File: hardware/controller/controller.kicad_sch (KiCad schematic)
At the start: 4 parts

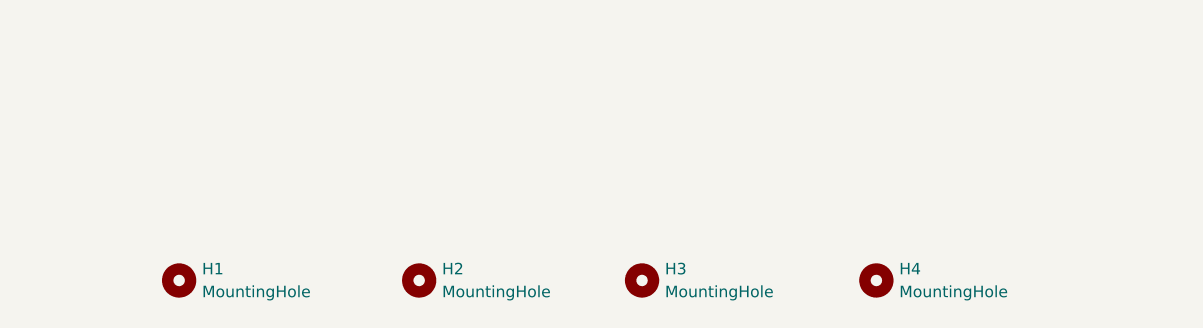
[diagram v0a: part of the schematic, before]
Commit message: hooking up parts in the schematic
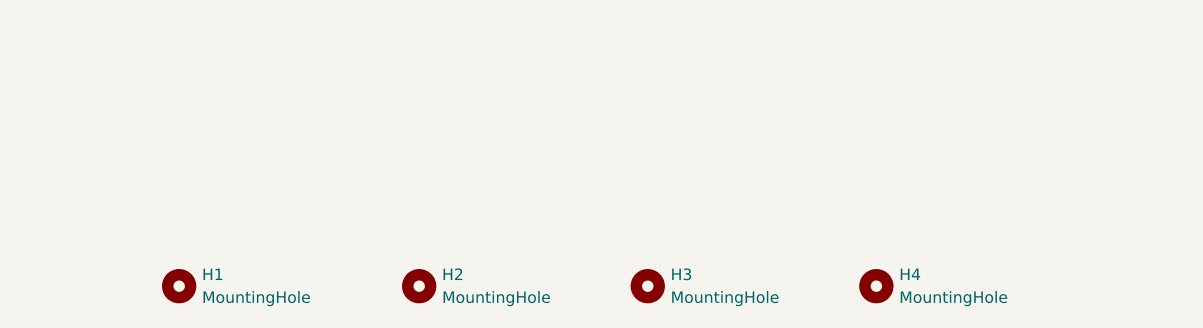
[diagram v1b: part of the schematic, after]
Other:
- moved on the sheet: H1, H2, H3, H4
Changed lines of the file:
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@@
 	(symbol
 		(lib_id "Mechanical:MountingHole")
-		(at 48.26 102.235 0)
+		(at 48.26 102.87 0)
 		(unit 1)
 		(body_style 1)
@@
 		(fields_autoplaced yes)
 		(property "Reference" "H1"
-			(at 50.8 100.9649 0)
-			(show_name no)
-			(do_not_autoplace no)
-			(effects
-				(font
-					(size 1.27 1.27)
-				)
-				(justify left)
-			)
-		)
-		(property "Value" "MountingHole"
-			(at 50.8 103.5049 0)
-			(show_name no)
-			(do_not_autoplace no)
-			(effects
-				(font
-					(size 1.27 1.27)
-				)
-				(justify left)
-			)
-		)
-		(property "Footprint" "MountingHole:MountingHole_3.2mm_M3_Pad"
-			(at 48.26 102.235 0)
-			(hide yes)
-			(show_name no)
-			(do_not_autoplace no)
-			(effects
-				(font
-					(size 1.27 1.27)
-				)
-			)
-		)
-		(property "Datasheet" ""
-			(at 48.26 102.235 0)
-			(hide yes)
-			(show_name no)
-			(do_not_autoplace no)
-			(effects
-				(font
-					(size 1.27 1.27)
-				)
-			)
-		)
-		(property "Description" "Mounting Hole without connection"
-			(at 48.26 102.235 0)
+			(at 50.8 101.5999 0)
+			(show_name no)
+			(do_not_autoplace no)
+			(effects
+				(font
+					(size 1.27 1.27)
+				)
+				(justify left)
+			)
+		)
+		(property "Value" "MountingHole"
+			(at 50.8 104.1399 0)
+			(show_name no)
+			(do_not_autoplace no)
+			(effects
+				(font
+					(size 1.27 1.27)
+				)
+				(justify left)
+			)
+		)
+		(property "Footprint" "MountingHole:MountingHole_3.2mm_M3_Pad"
+			(at 48.26 102.87 0)
+			(hide yes)
+			(show_name no)
+			(do_not_autoplace no)
+			(effects
+				(font
+					(size 1.27 1.27)
+				)
+			)
+		)
+		(property "Datasheet" ""
+			(at 48.26 102.87 0)
+			(hide yes)
+			(show_name no)
+			(do_not_autoplace no)
+			(effects
+				(font
+					(size 1.27 1.27)
+				)
+			)
+		)
+		(property "Description" "Mounting Hole without connection"
+			(at 48.26 102.87 0)
 			(hide yes)
 			(show_name no)
@@
 	(symbol
 		(lib_id "Mechanical:MountingHole")
-		(at 125.73 102.235 0)
+		(at 125.73 102.87 0)
 		(unit 1)
 		(body_style 1)
@@
 		(fields_autoplaced yes)
 		(property "Reference" "H4"
-			(at 128.27 100.9649 0)
-			(show_name no)
-			(do_not_autoplace no)
-			(effects
-				(font
-					(size 1.27 1.27)
-				)
-				(justify left)
-			)
-		)
-		(property "Value" "MountingHole"
-			(at 128.27 103.5049 0)
-			(show_name no)
-			(do_not_autoplace no)
-			(effects
-				(font
-					(size 1.27 1.27)
-				)
-				(justify left)
-			)
-		)
-		(property "Footprint" "MountingHole:MountingHole_3.2mm_M3_Pad"
-			(at 125.73 102.235 0)
-			(hide yes)
-			(show_name no)
-			(do_not_autoplace no)
-			(effects
-				(font
-					(size 1.27 1.27)
-				)
-			)
-		)
-		(property "Datasheet" ""
-			(at 125.73 102.235 0)
-			(hide yes)
-			(show_name no)
-			(do_not_autoplace no)
-			(effects
-				(font
-					(size 1.27 1.27)
-				)
-			)
-		)
-		(property "Description" "Mounting Hole without connection"
-			(at 125.73 102.235 0)
+			(at 128.27 101.5999 0)
+			(show_name no)
+			(do_not_autoplace no)
+			(effects
+				(font
+					(size 1.27 1.27)
+				)
+				(justify left)
+			)
+		)
+		(property "Value" "MountingHole"
+			(at 128.27 104.1399 0)
+			(show_name no)
+			(do_not_autoplace no)
+			(effects
+				(font
+					(size 1.27 1.27)
+				)
+				(justify left)
+			)
+		)
+		(property "Footprint" "MountingHole:MountingHole_3.2mm_M3_Pad"
+			(at 125.73 102.87 0)
+			(hide yes)
+			(show_name no)
+			(do_not_autoplace no)
+			(effects
+				(font
+					(size 1.27 1.27)
+				)
+			)
+		)
+		(property "Datasheet" ""
+			(at 125.73 102.87 0)
+			(hide yes)
+			(show_name no)
+			(do_not_autoplace no)
+			(effects
+				(font
+					(size 1.27 1.27)
+				)
+			)
+		)
+		(property "Description" "Mounting Hole without connection"
+			(at 125.73 102.87 0)
 			(hide yes)
 			(show_name no)
@@
 	(symbol
 		(lib_id "Mechanical:MountingHole")
-		(at 74.93 102.235 0)
+		(at 74.93 102.87 0)
 		(unit 1)
 		(body_style 1)
@@
 		(fields_autoplaced yes)
 		(property "Reference" "H2"
-			(at 77.47 100.9649 0)
-			(show_name no)
-			(do_not_autoplace no)
-			(effects
-				(font
-					(size 1.27 1.27)
-				)
-				(justify left)
-			)
-		)
-		(property "Value" "MountingHole"
-			(at 77.47 103.5049 0)
-			(show_name no)
-			(do_not_autoplace no)
-			(effects
-				(font
-					(size 1.27 1.27)
-				)
-				(justify left)
-			)
-		)
-		(property "Footprint" "MountingHole:MountingHole_3.2mm_M3_Pad"
-			(at 74.93 102.235 0)
-			(hide yes)
-			(show_name no)
-			(do_not_autoplace no)
-			(effects
-				(font
-					(size 1.27 1.27)
-				)
-			)
-		)
-		(property "Datasheet" ""
-			(at 74.93 102.235 0)
-			(hide yes)
-			(show_name no)
-			(do_not_autoplace no)
-			(effects
-				(font
-					(size 1.27 1.27)
-				)
-			)
-		)
-		(property "Description" "Mounting Hole without connection"
-			(at 74.93 102.235 0)
+			(at 77.47 101.5999 0)
+			(show_name no)
+			(do_not_autoplace no)
+			(effects
+				(font
+					(size 1.27 1.27)
+				)
+				(justify left)
+			)
+		)
+		(property "Value" "MountingHole"
+			(at 77.47 104.1399 0)
+			(show_name no)
+			(do_not_autoplace no)
+			(effects
+				(font
+					(size 1.27 1.27)
+				)
+				(justify left)
+			)
+		)
+		(property "Footprint" "MountingHole:MountingHole_3.2mm_M3_Pad"
+			(at 74.93 102.87 0)
+			(hide yes)
+			(show_name no)
+			(do_not_autoplace no)
+			(effects
+				(font
+					(size 1.27 1.27)
+				)
+			)
+		)
+		(property "Datasheet" ""
+			(at 74.93 102.87 0)
+			(hide yes)
+			(show_name no)
+			(do_not_autoplace no)
+			(effects
+				(font
+					(size 1.27 1.27)
+				)
+			)
+		)
+		(property "Description" "Mounting Hole without connection"
+			(at 74.93 102.87 0)
 			(hide yes)
 			(show_name no)
@@
 	(symbol
 		(lib_id "Mechanical:MountingHole")
-		(at 99.695 102.235 0)
+		(at 100.33 102.87 0)
 		(unit 1)
 		(body_style 1)
@@
 		(fields_autoplaced yes)
 		(property "Reference" "H3"
-			(at 102.235 100.9649 0)
-			(show_name no)
-			(do_not_autoplace no)
-			(effects
-				(font
-					(size 1.27 1.27)
-				)
-				(justify left)
-			)
-		)
-		(property "Value" "MountingHole"
-			(at 102.235 103.5049 0)
-			(show_name no)
-			(do_not_autoplace no)
-			(effects
-				(font
-					(size 1.27 1.27)
-				)
-				(justify left)
-			)
-		)
-		(property "Footprint" "MountingHole:MountingHole_3.2mm_M3_Pad"
-			(at 99.695 102.235 0)
-			(hide yes)
-			(show_name no)
-			(do_not_autoplace no)
-			(effects
-				(font
-					(size 1.27 1.27)
-				)
-			)
-		)
-		(property "Datasheet" ""
-			(at 99.695 102.235 0)
-			(hide yes)
-			(show_name no)
-			(do_not_autoplace no)
-			(effects
-				(font
-					(size 1.27 1.27)
-				)
-			)
-		)
-		(property "Description" "Mounting Hole without connection"
-			(at 99.695 102.235 0)
-			(hide yes)
-			(show_name no)
+			(at 102.87 101.5999 0)
+			(show_name no)
+			(do_not_autoplace no)
+			(effects
+				(font
+					(size 1.27 1.27)
+				)
+				(justify left)
+			)
+		)
+		(property "Value" "MountingHole"
+			(at 102.87 104.1399 0)
+			(show_name no)
+			(do_not_autoplace no)
+			(effects
+				(font
+					(size 1.27 1.27)
+				)
+				(justify left)
+			)
+		)
+		(property "Footprint" "MountingHole:MountingHole_3.2mm_M3_Pad"
+			(at 100.33 102.87 0)
+			(hide yes)
+			(show_name no)
+			(do_not_autoplace no)
+			(effects
+				(font
+					(size 1.27 1.27)
+				)
+			)
+		)
+		(property "Datasheet" ""
+			(at 100.33 102.87 0)
+			(hide yes)
+			(show_name no)
+			(do_not_autoplace no)
+			(effects
+				(font
+					(size 1.27 1.27)
+				)
+			)
+		)
+		(property "Description" "Mounting Hole without connection"
+			(at 100.33 102.87 0)
+			(hide yes)
+			(show_name no)
